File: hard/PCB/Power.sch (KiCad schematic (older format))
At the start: 47 parts, among them P2 CONN_02X03, U2 TPS62133RGTR, U3 ZLDO1117G33TA, U4 ZLDO1117G12TA

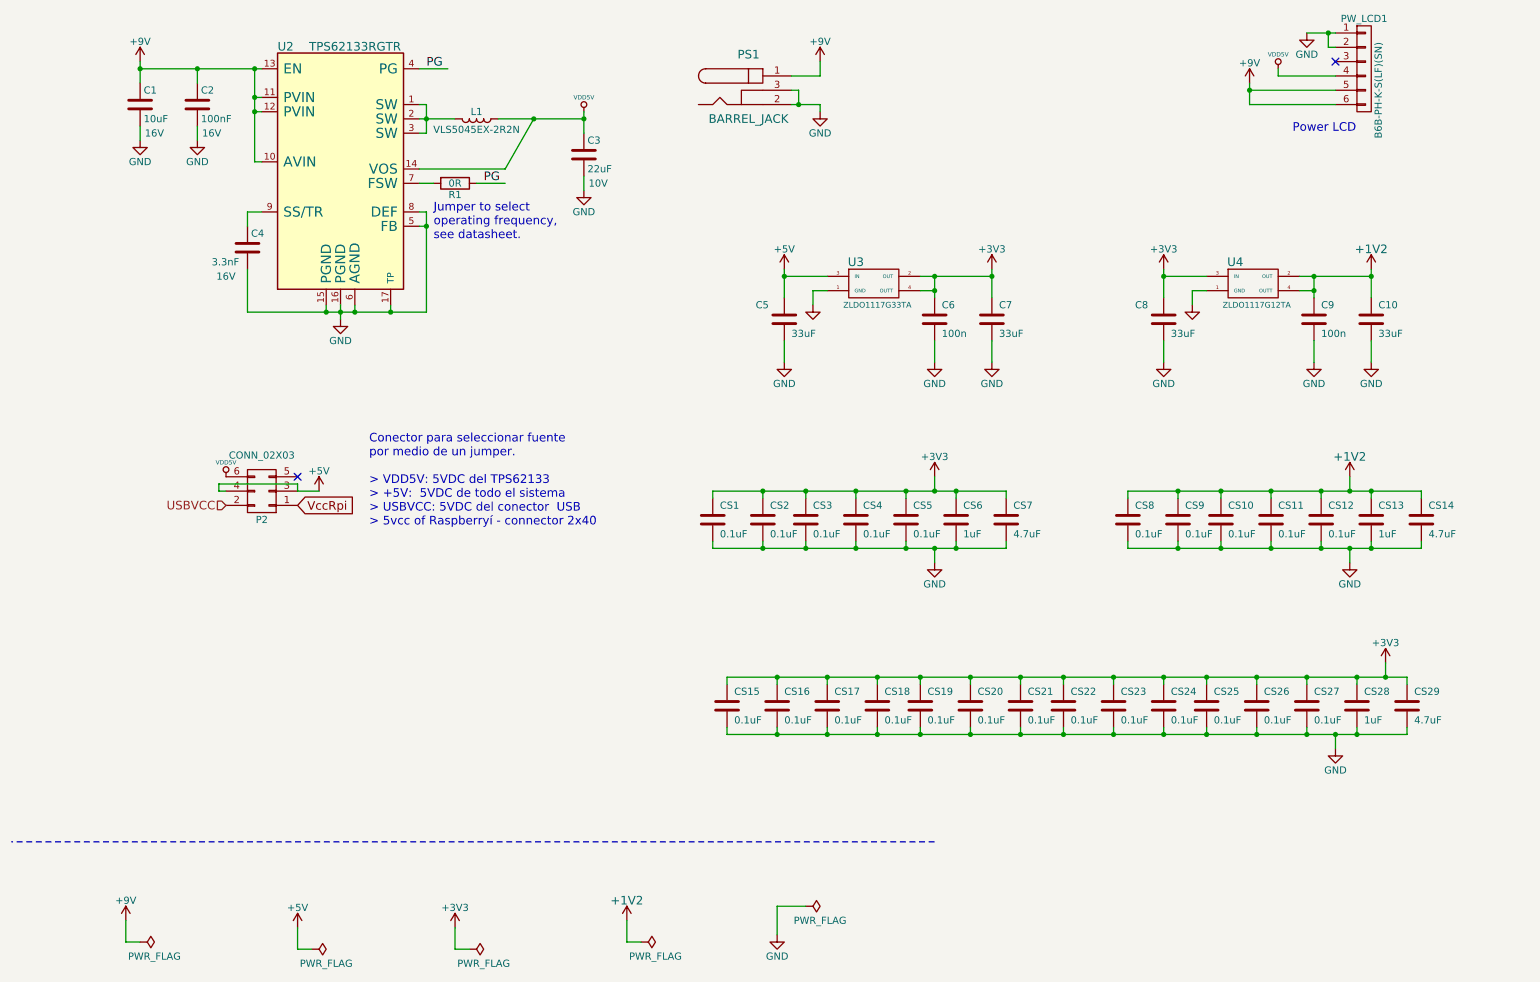
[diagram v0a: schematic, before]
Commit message: Changes in HDMISpartan6_Board
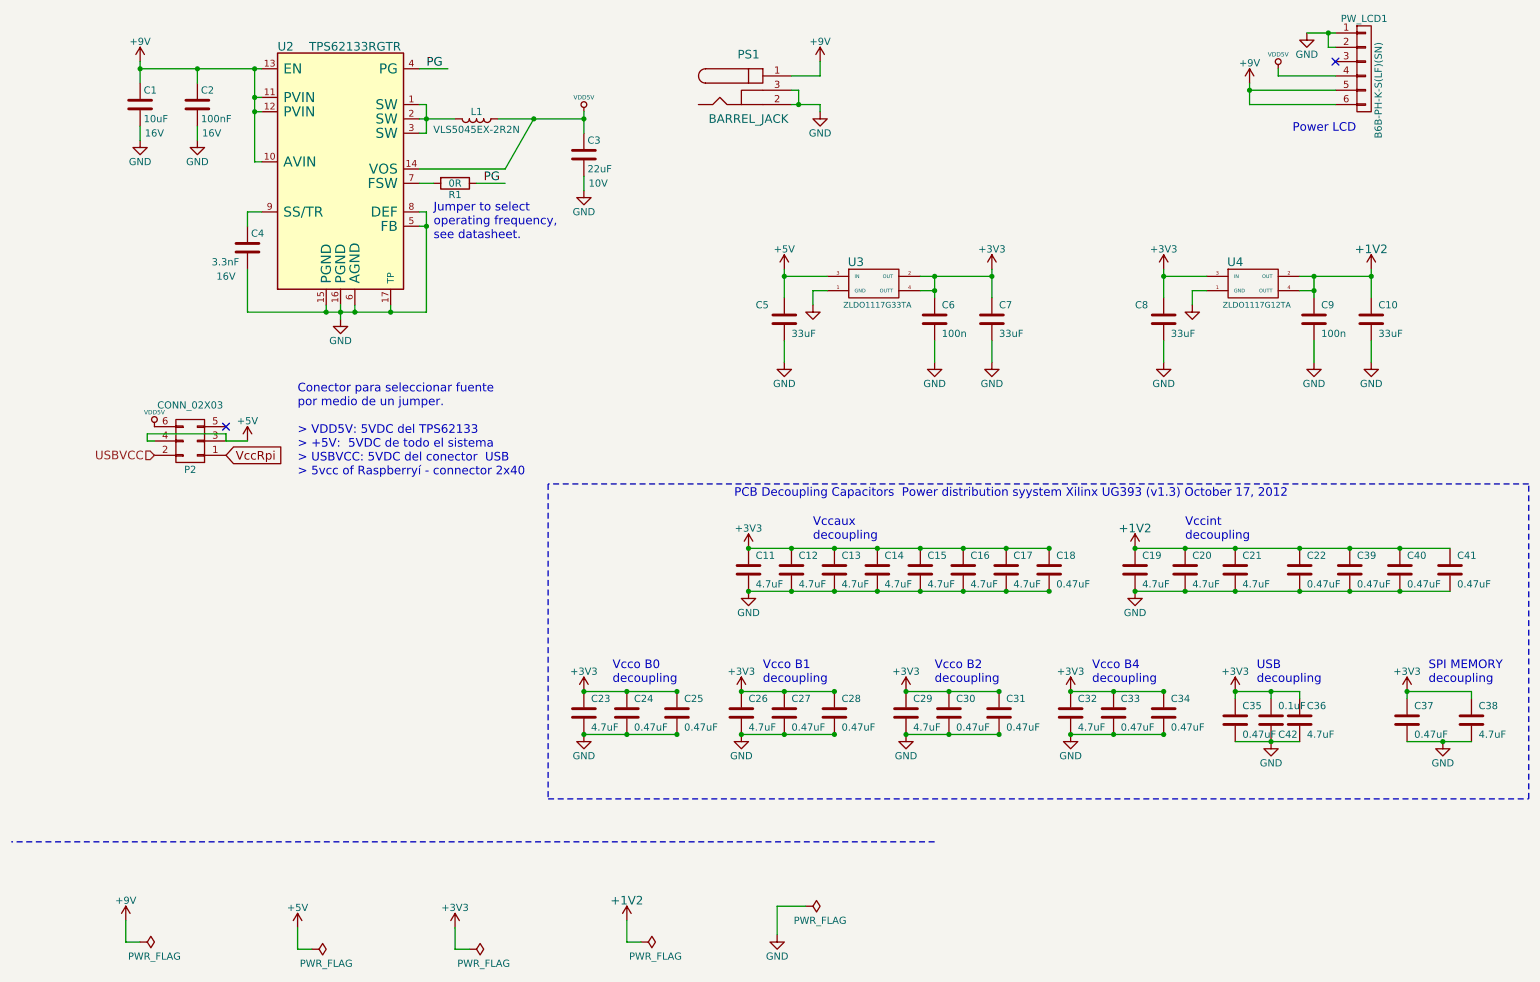
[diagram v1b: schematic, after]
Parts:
- removed CS1, CS10, CS11, CS12, CS15, CS16, CS17, CS18, CS19, CS2, CS20, CS21, CS22, CS23, CS24, CS25, CS26, CS27, CS3, CS4, CS5, CS8, CS9: 0.1uF, Capacitors_SMD:C_0603, symbol C
- removed CS13, CS28, CS6: 1uF, Capacitors_SMD:C_0603, symbol C
- removed CS29, CS7: 4.7uF, Capacitors_SMD:C_1206, symbol C
- added C11, C12, C13, C14, C15, C16, C17, C19, C20, C21, C23, C26, C29, C32, C38: 4.7uF, Capacitors_SMD:C_0805, symbol C
- added C18, C22, C24, C25, C27, C28, C30, C31, C33, C34, C35, C37, C39, C40, C41: 0.47uF, Capacitors_SMD:C_0402, symbol C
- added C42: 0.1uF, Capacitors_SMD:C_0603, symbol C
- C36: renamed from CS14; footprint Capacitors_SMD:C_1206 -> Capacitors_SMD:C_0805; DIGIKEY REF (none) -> Ceramic X5R ESR < 60mOhm
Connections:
- net +1V2: now also C19.1, C20.1, C21.1, C22.1, C39.1, C40.1, C41.1; no longer C36.1
- net +3V3: now also C36.1, C11.1, C12.1, C13.1, C14.1, C15.1, C16.1, C17.1, C18.1, C23.1, C24.1, C25.1, C26.1, C27.1, C28.1, C29.1, C30.1, C31.1, C32.1, C33.1, C34.1, C35.1, C37.1, C38.1, C42.2
- net GND: now also C11.2, C12.2, C13.2, C14.2, C15.2, C16.2, C17.2, C18.2, C19.2, C20.2, C21.2, C22.2, C23.2, C24.2, C25.2, C26.2, C27.2, C28.2, C29.2, C30.2, C31.2, C32.2, C33.2, C34.2, C35.2, C37.2, C38.2, C39.2, C40.2, C41.2, C42.1
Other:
- note added: "PCB Decoupling Capacitors Power distribution syystem Xilinx UG393 (v1.3) October 17, 2012"
- note added: "SPI MEMORY\ndecoupling"
- note added: "USB \ndecoupling"
- note added: "Vccaux\ndecoupling"
- note added: "Vccint \ndecoupling"
- note added: "Vcco B0\ndecoupling"
- note added: "Vcco B1\ndecoupling"
- note added: "Vcco B2\ndecoupling"
- note added: "Vcco B4\ndecoupling"
- moved on the sheet: C36, P2
